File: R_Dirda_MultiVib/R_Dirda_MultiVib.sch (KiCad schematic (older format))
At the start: 10 parts, among them U1 DMC20101

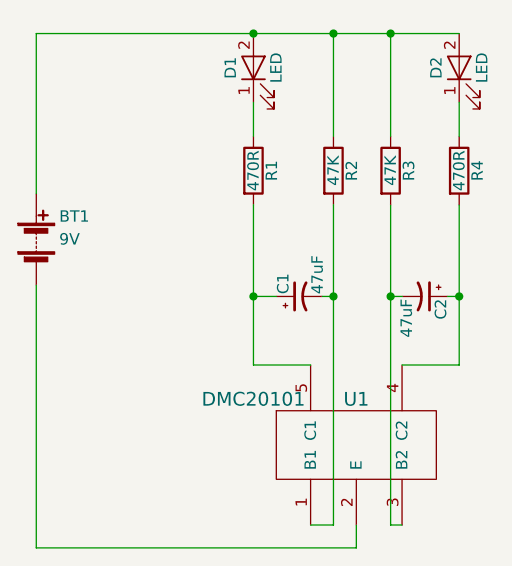
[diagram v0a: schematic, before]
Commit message: 0.22
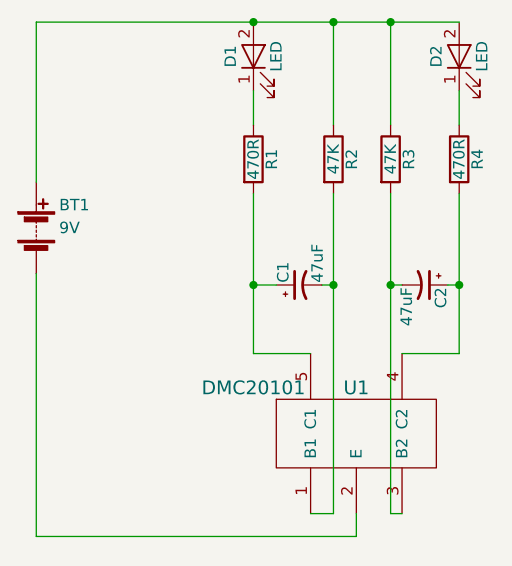
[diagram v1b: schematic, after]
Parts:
- U1: footprint (none) -> TO_SOT_Packages_SMD:SOT-23-5
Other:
- moved on the sheet: BT1, C1, C2, D1, D2, R1, R2, R3, R4, U1
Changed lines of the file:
@@
 L LED D1
 U 1 1 5A8E904A
-P 2650 2750
-F 0 "D1" H 2650 2850 50  0000 C CNN
-F 1 "LED" H 2650 2650 50  0000 C CNN
-F 2 "" H 2650 2750 50  0001 C CNN
-F 3 "" H 2650 2750 50  0001 C CNN
-	1    2650 2750
+P 2650 2700
+F 0 "D1" H 2650 2800 50  0000 C CNN
+F 1 "LED" H 2650 2600 50  0000 C CNN
+F 2 "" H 2650 2700 50  0001 C CNN
+F 3 "" H 2650 2700 50  0001 C CNN
+	1    2650 2700
 	0    -1   -1   0
 $EndComp
@@
 L LED D2
 U 1 1 5A8E90A6
-P 3550 2750
-F 0 "D2" H 3550 2850 50  0000 C CNN
-F 1 "LED" H 3550 2650 50  0000 C CNN
-F 2 "" H 3550 2750 50  0001 C CNN
-F 3 "" H 3550 2750 50  0001 C CNN
-	1    3550 2750
+P 3550 2700
+F 0 "D2" H 3550 2800 50  0000 C CNN
+F 1 "LED" H 3550 2600 50  0000 C CNN
+F 2 "" H 3550 2700 50  0001 C CNN
+F 3 "" H 3550 2700 50  0001 C CNN
+	1    3550 2700
 	0    -1   -1   0
 $EndComp
@@
 L R R1
 U 1 1 5A8E915E
-P 2650 3200
-F 0 "R1" V 2730 3200 50  0000 C CNN
-F 1 "470R" V 2650 3200 50  0000 C CNN
-F 2 "" V 2580 3200 50  0001 C CNN
-F 3 "" H 2650 3200 50  0001 C CNN
-	1    2650 3200
+P 2650 3150
+F 0 "R1" V 2730 3150 50  0000 C CNN
+F 1 "470R" V 2650 3150 50  0000 C CNN
+F 2 "" V 2580 3150 50  0001 C CNN
+F 3 "" H 2650 3150 50  0001 C CNN
+	1    2650 3150
 	1    0    0    -1
 $EndComp
@@
 L R R2
 U 1 1 5A8E91B0
-P 3000 3200
-F 0 "R2" V 3080 3200 50  0000 C CNN
-F 1 "47K" V 3000 3200 50  0000 C CNN
-F 2 "" V 2930 3200 50  0001 C CNN
-F 3 "" H 3000 3200 50  0001 C CNN
-	1    3000 3200
+P 3000 3150
+F 0 "R2" V 3080 3150 50  0000 C CNN
+F 1 "47K" V 3000 3150 50  0000 C CNN
+F 2 "" V 2930 3150 50  0001 C CNN
+F 3 "" H 3000 3150 50  0001 C CNN
+	1    3000 3150
 	1    0    0    -1
 $EndComp
@@
 L R R3
 U 1 1 5A8E91F7
-P 3250 3200
-F 0 "R3" V 3330 3200 50  0000 C CNN
-F 1 "47K" V 3250 3200 50  0000 C CNN
-F 2 "" V 3180 3200 50  0001 C CNN
-F 3 "" H 3250 3200 50  0001 C CNN
-	1    3250 3200
+P 3250 3150
+F 0 "R3" V 3330 3150 50  0000 C CNN
+F 1 "47K" V 3250 3150 50  0000 C CNN
+F 2 "" V 3180 3150 50  0001 C CNN
+F 3 "" H 3250 3150 50  0001 C CNN
+	1    3250 3150
 	1    0    0    -1
 $EndComp
@@
 L R R4
 U 1 1 5A8E922C
-P 3550 3200
-F 0 "R4" V 3630 3200 50  0000 C CNN
-F 1 "470R" V 3550 3200 50  0000 C CNN
-F 2 "" V 3480 3200 50  0001 C CNN
-F 3 "" H 3550 3200 50  0001 C CNN
-	1    3550 3200
+P 3550 3150
+F 0 "R4" V 3630 3150 50  0000 C CNN
+F 1 "470R" V 3550 3150 50  0000 C CNN
+F 2 "" V 3480 3150 50  0001 C CNN
+F 3 "" H 3550 3150 50  0001 C CNN
+	1    3550 3150
 	1    0    0    -1
 $EndComp
@@
 L Battery BT1
 U 1 1 5A8E9273
-P 1700 3500
-F 0 "BT1" H 1800 3600 50  0000 L CNN
-F 1 "9V" H 1800 3500 50  0000 L CNN
-F 2 "" V 1700 3560 50  0001 C CNN
-F 3 "" V 1700 3560 50  0001 C CNN
-	1    1700 3500
+P 1700 3450
+F 0 "BT1" H 1800 3550 50  0000 L CNN
+F 1 "9V" H 1800 3450 50  0000 L CNN
+F 2 "" V 1700 3510 50  0001 C CNN
+F 3 "" V 1700 3510 50  0001 C CNN
+	1    1700 3450
 	1    0    0    -1
 $EndComp
@@
 L CP1_Small C1
 U 1 1 5A8E92BC
-P 2850 3750
-F 0 "C1" H 2860 3820 50  0000 L CNN
-F 1 "47uF" H 2860 3670 50  0000 L CNN
-F 2 "" H 2850 3750 50  0001 C CNN
-F 3 "" H 2850 3750 50  0001 C CNN
-	1    2850 3750
+P 2850 3700
+F 0 "C1" H 2860 3770 50  0000 L CNN
+F 1 "47uF" H 2860 3620 50  0000 L CNN
+F 2 "" H 2850 3700 50  0001 C CNN
+F 3 "" H 2850 3700 50  0001 C CNN
+	1    2850 3700
 	0    -1   -1   0
 $EndComp
@@
 L CP1_Small C2
 U 1 1 5A8E9336
-P 3400 3750
-F 0 "C2" H 3410 3820 50  0000 L CNN
-F 1 "47uF" H 3410 3670 50  0000 L CNN
-F 2 "" H 3400 3750 50  0001 C CNN
-F 3 "" H 3400 3750 50  0001 C CNN
-	1    3400 3750
+P 3400 3700
+F 0 "C2" H 3410 3770 50  0000 L CNN
+F 1 "47uF" H 3410 3620 50  0000 L CNN
+F 2 "" H 3400 3700 50  0001 C CNN
+F 3 "" H 3400 3700 50  0001 C CNN
+	1    3400 3700
 	0    1    1    0
 $EndComp
 Wire Wire Line
-	2650 2900 2650 3050
+	2650 2850 2650 3000
 Wire Wire Line
-	2650 3350 2650 4050
+	2650 3300 2650 4000
 Wire Wire Line
-	2750 3750 2650 3750
-Connection ~ 2650 3750
+	2750 3700 2650 3700
+Connection ~ 2650 3700
 Wire Wire Line
-	1700 2600 3550 2600
+	1700 2550 3550 2550
 Wire Wire Line
-	3000 3050 3000 2600
-Connection ~ 3000 2600
+	3000 3000 3000 2550
+Connection ~ 3000 2550
 Wire Wire Line
-	3550 3050 3550 2900
+	3550 3000 3550 2850
 Wire Wire Line
-	2950 3750 3000 3750
+	2950 3700 3000 3700
 Wire Wire Line
-	3000 3350 3000 4750
+	3000 3300 3000 4700
 Wire Wire Line
-	1700 2600 1700 3300
-Connection ~ 2650 2600
+	1700 2550 1700 3250
+Connection ~ 2650 2550
 Wire Wire Line
-	1700 3700 1700 4850
+	1700 3650 1700 4800
 Wire Wire Line
-	3250 3050 3250 2600
-Connection ~ 3250 2600
+	3250 3000 3250 2550
+Connection ~ 3250 2550
 Wire Wire Line
-	3250 3350 3250 4750
+	3250 3300 3250 4700
 Wire Wire Line
-	3550 3350 3550 4050
+	3550 3300 3550 4000
 Wire Wire Line
-	3550 3750 3500 3750
-Connection ~ 3250 3750
-Connection ~ 3000 3750
-Connection ~ 3550 3750
+	3550 3700 3500 3700
+Connection ~ 3250 3700
+Connection ~ 3000 3700
+Connection ~ 3550 3700
 $Comp
 L DMC20101 U1
 U 1 1 5AA94427
-P 3100 4400
-F 0 "U1" H 3100 4600 60  0000 C CNN
-F 1 "DMC20101" H 2650 4600 60  0000 C CNN
-F 2 "" H 2650 4600 60  0001 C CNN
-F 3 "" H 2650 4600 60  0001 C CNN
-	1    3100 4400
+P 3100 4350
+F 0 "U1" H 3100 4550 60  0000 C CNN
+F 1 "DMC20101" H 2650 4550 60  0000 C CNN
+F 2 "TO_SOT_Packages_SMD:SOT-23-5" H 2650 4550 60  0001 C CNN
+F 3 "" H 2650 4550 60  0001 C CNN
+	1    3100 4350
 	1    0    0    -1
 $EndComp
 Wire Wire Line
-	2650 4050 2900 4050
+	2650 4000 2900 4000
 Wire Wire Line
-	3550 4050 3300 4050
+	3550 4000 3300 4000
 Wire Wire Line
-	3000 4750 2900 4750
+	3000 4700 2900 4700
 Wire Wire Line
-	3250 4750 3300 4750
+	3250 4700 3300 4700
 Wire Wire Line
-	1700 4850 3100 4850
+	1700 4800 3100 4800
 Wire Wire Line
-	3100 4850 3100 4750
+	3100 4800 3100 4700
 Wire Wire Line
-	3300 3750 3250 3750
+	3300 3700 3250 3700
 $EndSCHEMATC
